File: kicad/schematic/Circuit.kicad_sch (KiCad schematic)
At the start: 54 parts, among them M1 Motor_DC, M2 Motor_DC, M3 Motor_DC, M4 Motor_DC, M5 Motor_DC, M6 Motor_DC, M7 Motor_DC, M8 Motor_DC, Q1 AO3400A, Q2 AO3400A, Q3 AO3400A, Q4 AO3400A, Q5 AO3400A, Q6 AO3400A, Q7 AO3400A, Q8 AO3400A

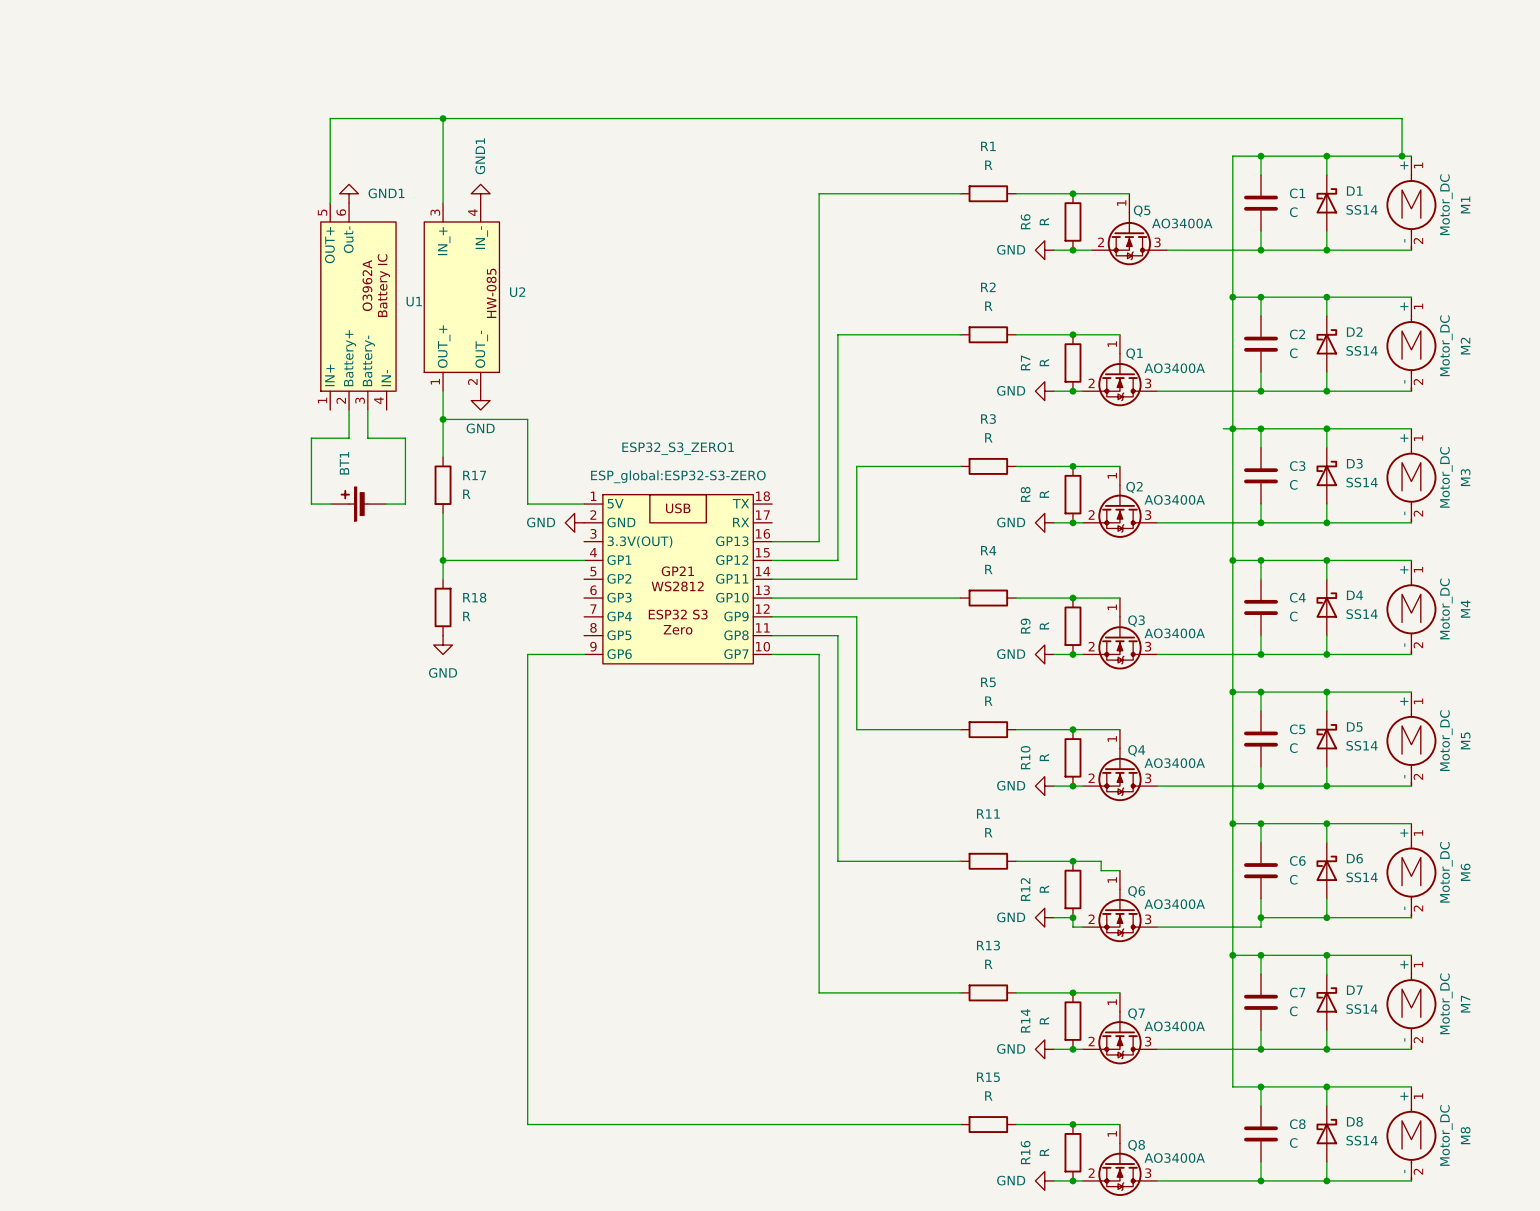
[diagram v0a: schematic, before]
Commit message: changed board layout. WIP
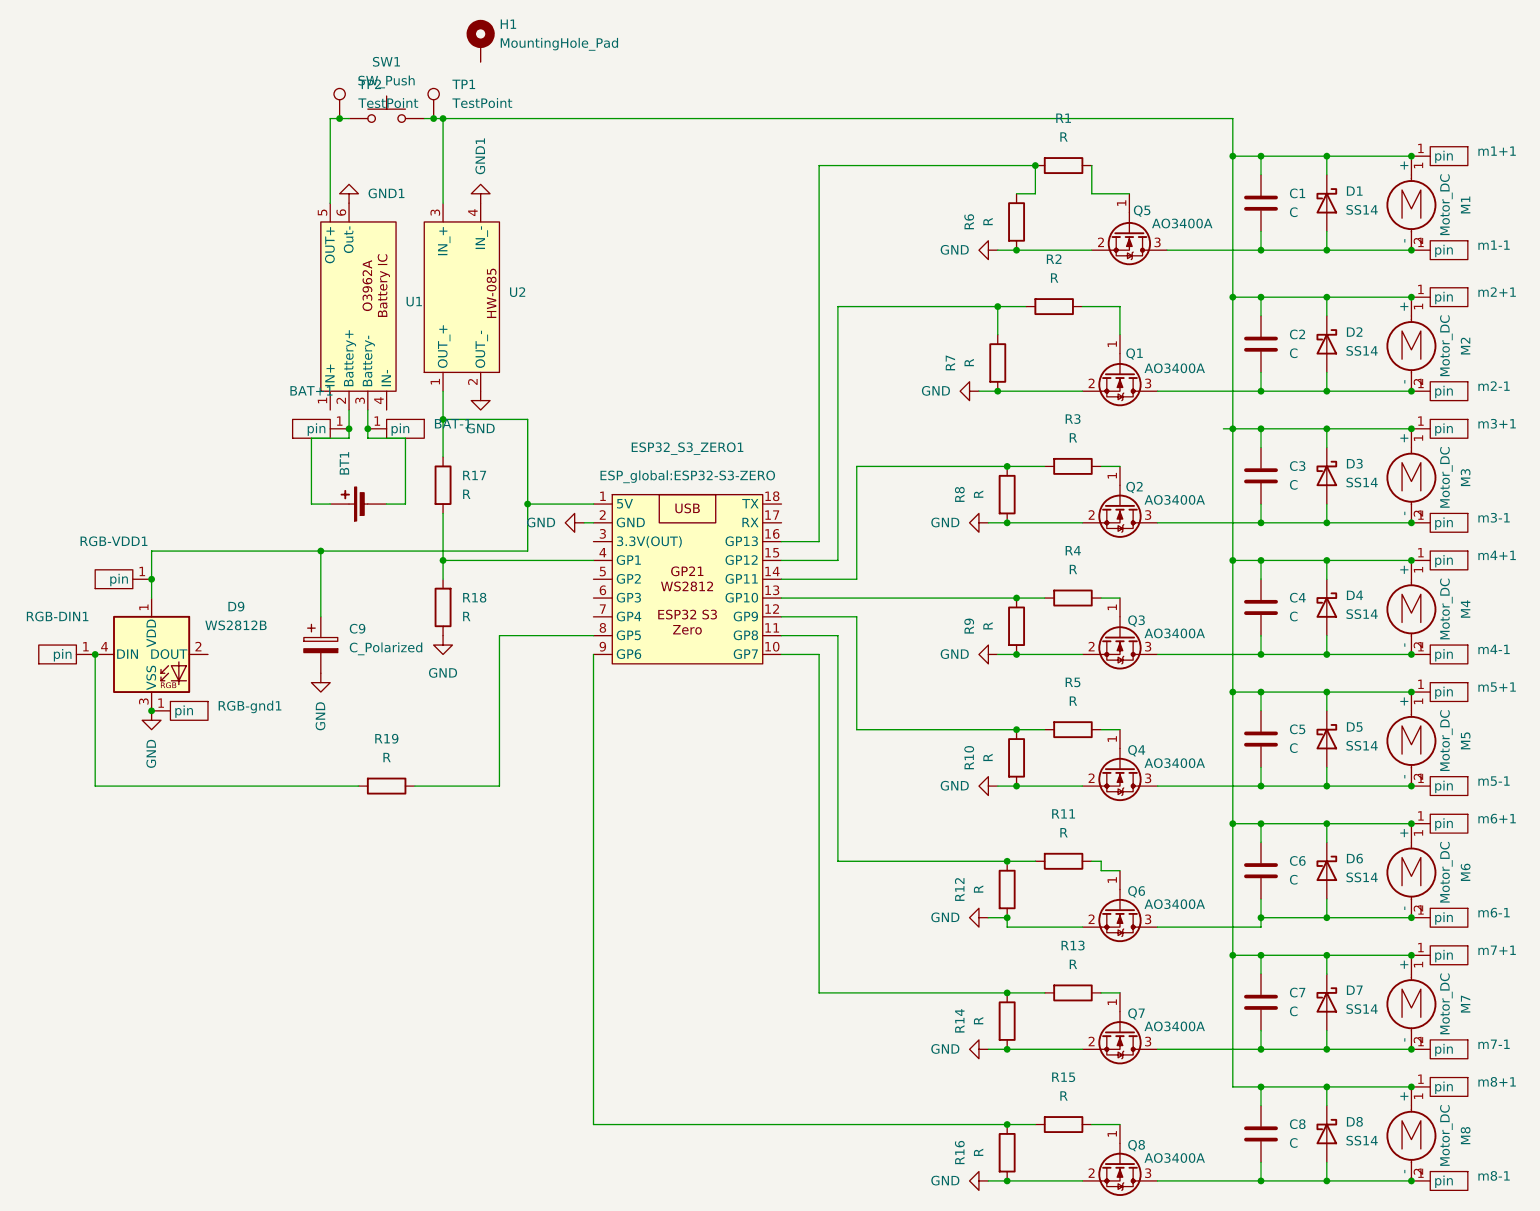
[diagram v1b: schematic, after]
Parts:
- added BAT+1, BAT-1, RGB-DIN1, RGB-VDD1, RGB-gnd1, m1+1, m1-1, m2+1, m2-1, m3+1, m3-1, m4+1, m4-1, m5+1, m5-1, m6+1, m6-1, m7+1, m7-1, m8+1, m8-1: ~, ESP_global:blank pad, symbol waveshare_esp32_s3_mini_zero:blank_pad_1
- added C9: C_Polarized, Capacitor_SMD:CP_Elec_8x10.5, symbol Device:C_Polarized
- added D9: WS2812B, LED_SMD:LED_WS2812B_PLCC4_5.0x5.0mm_P3.2mm, symbol LED:WS2812B
- added H1: MountingHole_Pad, symbol Mechanical:MountingHole_Pad
- added R19: R, Resistor_SMD:R_0805_2012Metric, symbol Device:R
- added SW1: SW_Push, symbol Switch:SW_Push
- added TP1, TP2: TestPoint, symbol Connector:TestPoint
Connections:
- net GND: now also C9.2, D9.3 (VSS), RGB-gnd1.1 (pin)
- net at C1.2, C2.2, C3.2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: now also SW1.2, TP1.1, m1+1.1 (pin), m2+1.1 (pin), m3+1.1 (pin), m4+1.1 (pin), m5+1.1 (pin), m6+1.1 (pin), m7+1.1 (pin), m8+1.1 (pin); no longer U1.5 (OUT+)
- net at C2.1, D2.2 (A), M2.2 (-)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: now also m2-1.1 (pin)
- net at BT1.1 (+), U1.2 (Battery+): now also BAT+1.1 (pin)
- net at BT1.2 (-), U1.3 (Battery-): now also BAT-1.1 (pin)
- net at C8.1, D8.2 (A), M8.2 (-)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: now also m8-1.1 (pin)
- net at Q3.1 (G), R4.1: no longer R9.1
- net at C4.1, D4.2 (A), M4.2 (-)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: now also m4-1.1 (pin)
- net at ESP32_S3_ZERO1.13 (GP10), R4.2: now also R9.1
- net at Q6.1 (G), R11.1: no longer R12.1
- net at C6.1, D6.2 (A), M6.2 (-)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: now also m6-1.1 (pin)
- net at Q7.1 (G), R13.1: no longer R14.1
- net at C5.1, D5.2 (A), M5.2 (-)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: now also m5-1.1 (pin)
- net at Q4.1 (G), R5.1: no longer R10.1
- net at ESP32_S3_ZERO1.12 (GP9), R5.2: now also R10.1
- net at Q8.1 (G), R15.1: no longer R16.1
- net at ESP32_S3_ZERO1.9 (GP6), R15.2: now also R16.1
- net at Q5.1 (G), R1.1: no longer R6.1
- net at C1.1, D1.2 (A), M1.2 (-)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: now also m1-1.1 (pin)
- net at Q1.1 (G), R2.1: no longer R7.1
- net at ESP32_S3_ZERO1.15 (GP12), R2.2: now also R7.1
- net at ESP32_S3_ZERO1.1 (5V), R17.1, U2.1 (OUT_+): now also C9.1, D9.1 (VDD), RGB-VDD1.1 (pin)
- net at C7.1, D7.2 (A), M7.2 (-)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: now also m7-1.1 (pin)
- net at Q2.1 (G), R3.1: no longer R8.1
- net at C3.1, D3.2 (A), M3.2 (-)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: now also m3-1.1 (pin)
- net at ESP32_S3_ZERO1.10 (GP7), R13.2: now also R14.1
- net at ESP32_S3_ZERO1.16 (GP13), R1.2: now also R6.1
- net at ESP32_S3_ZERO1.11 (GP8), R11.2: now also R12.1
- net at ESP32_S3_ZERO1.14 (GP11), R3.2: now also R8.1
- net at ESP32_S3_ZERO1.8 (GP5): now also R19.1
- new net: D9.4 (DIN), R19.2, RGB-DIN1.1 (pin)
- new net: SW1.1, TP2.1, U1.5 (OUT+)
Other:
- moved on the sheet: ESP32_S3_ZERO1, R1, R10, R11, R12, R13, R14, R15, R16, R2, R3, R4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
